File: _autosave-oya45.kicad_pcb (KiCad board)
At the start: 2 copper layers, 24 parts, among them SW1 SW_Push, U1 ATmega32U4-AU, Y1 16MHz

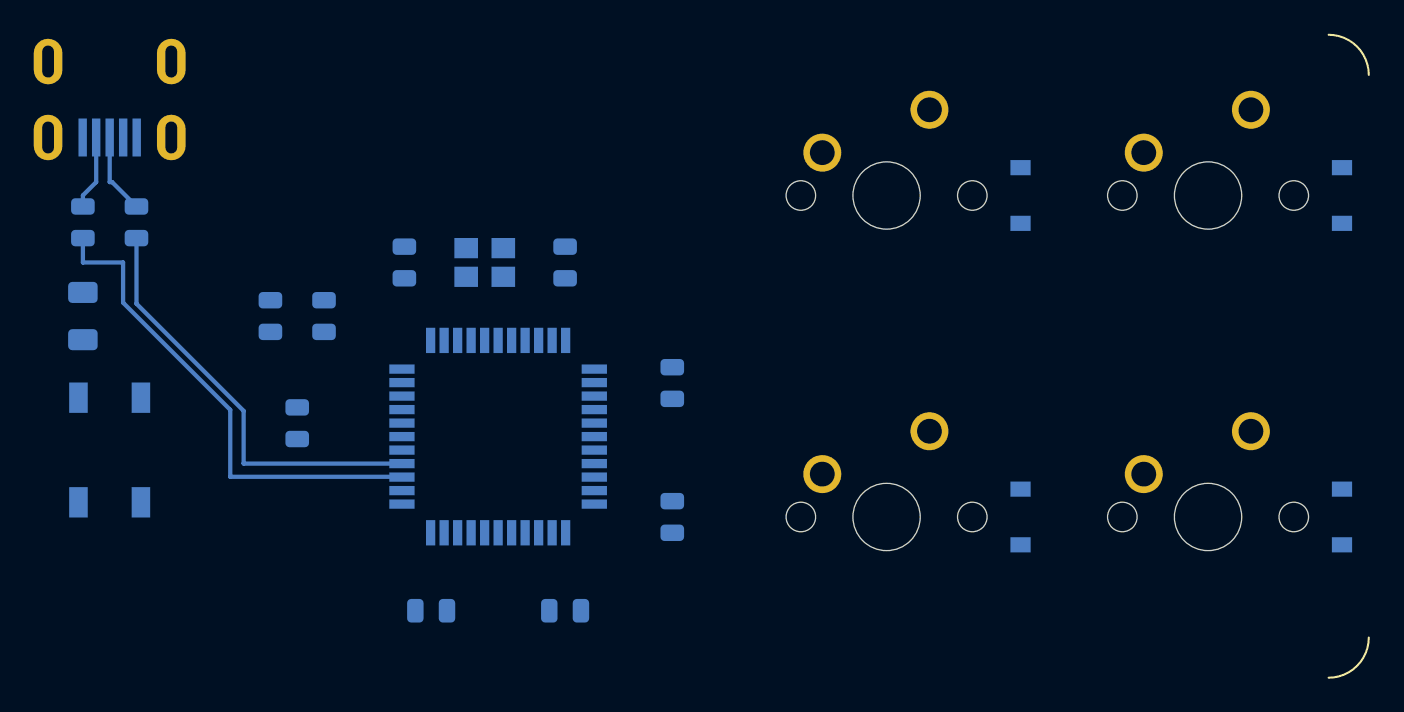
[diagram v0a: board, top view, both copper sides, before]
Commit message: test finish
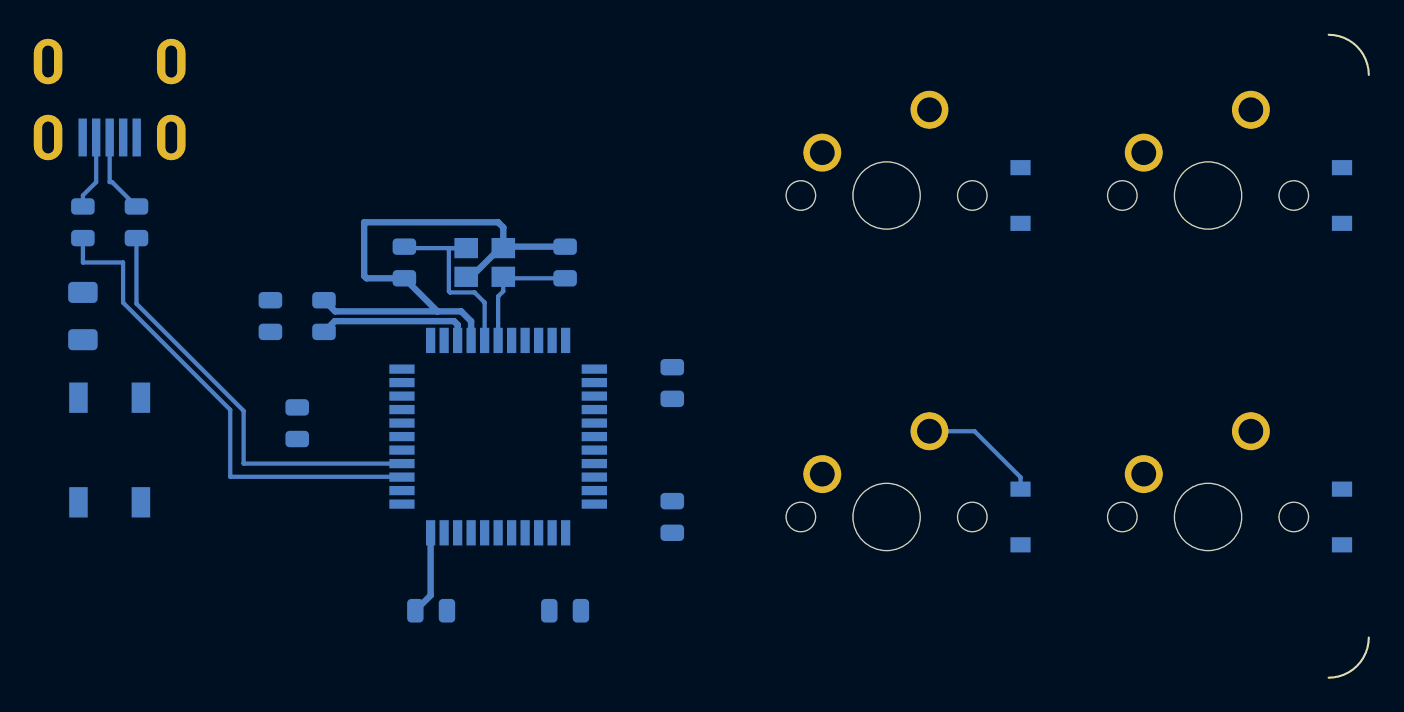
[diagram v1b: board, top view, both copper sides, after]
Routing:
- net GND: track 0.00 -> 35.0 mm
- net +5V: track 0.00 -> 14.2 mm
- net Net-(C3-Pad1): track 0.00 -> 11.9 mm
- net Net-(C2-Pad1): track 0.00 -> 7.59 mm
- net Net-(D3-Pad2): track 0.00 -> 7.23 mm
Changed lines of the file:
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@@
     (thickness 1.6)
     (drawings 2)
-    (tracks 17)
+    (tracks 58)
     (zones 0)
     (modules 24)
@@
   (gr_arc (start 194.46875 115.09375) (end 194.46875 117.475) (angle -90) (layer F.SilkS) (width 0.12))
   (gr_arc (start 194.46875 81.75625) (end 196.85 81.75625) (angle -90) (layer F.SilkS) (width 0.12))
+  (segment (start 145.5625 90.79375) (end 145.5625 92.01875) (width 0.381) (layer B.Cu) (net 1))
+  (segment (start 145.25625 90.4875) (end 145.5625 90.79375) (width 0.381) (layer B.Cu) (net 1))
+  (segment (start 137.31875 90.4875) (end 145.25625 90.4875) (width 0.381) (layer B.Cu) (net 1))
+  (segment (start 137.31875 93.6625) (end 137.31875 90.4875) (width 0.381) (layer B.Cu) (net 1))
+  (segment (start 139.7 93.80625) (end 137.4625 93.80625) (width 0.381) (layer B.Cu) (net 1))
+  (segment (start 137.4625 93.80625) (end 137.31875 93.6625) (width 0.381) (layer B.Cu) (net 1))
+  (segment (start 143.65625 96.3565) (end 143.65625 97.4875) (width 0.381) (layer B.Cu) (net 1))
+  (segment (start 145.65 91.93125) (end 145.5625 92.01875) (width 0.381) (layer B.Cu) (net 1))
+  (segment (start 149.225 91.93125) (end 145.65 91.93125) (width 0.381) (layer B.Cu) (net 1))
+  (segment (start 143.665402 93.71875) (end 143.3625 93.71875) (width 0.381) (layer B.Cu) (net 1))
+  (segment (start 145.365402 92.01875) (end 143.665402 93.71875) (width 0.381) (layer B.Cu) (net 1))
+  (segment (start 145.5625 92.01875) (end 145.365402 92.01875) (width 0.381) (layer B.Cu) (net 1))
+  (segment (start 143.065739 95.765989) (end 143.65625 96.3565) (width 0.381) (layer B.Cu) (net 1))
+  (segment (start 141.659739 95.765989) (end 143.065739 95.765989) (width 0.381) (layer B.Cu) (net 1))
+  (segment (start 139.7 93.80625) (end 141.659739 95.765989) (width 0.381) (layer B.Cu) (net 1))
+  (segment (start 135.597239 95.765989) (end 141.659739 95.765989) (width 0.381) (layer B.Cu) (net 1))
+  (segment (start 134.9375 95.10625) (end 135.597239 95.765989) (width 0.381) (layer B.Cu) (net 1))
+  (segment (start 142.85625 96.559598) (end 142.85625 97.4875) (width 0.381) (layer B.Cu) (net 2))
+  (segment (start 142.643651 96.346999) (end 142.85625 96.559598) (width 0.381) (layer B.Cu) (net 2))
+  (segment (start 135.571751 96.346999) (end 142.643651 96.346999) (width 0.381) (layer B.Cu) (net 2))
+  (segment (start 134.9375 96.98125) (end 135.571751 96.346999) (width 0.381) (layer B.Cu) (net 2))
+  (segment (start 141.25625 112.6) (end 140.35 113.50625) (width 0.381) (layer B.Cu) (net 2))
+  (segment (start 141.25625 108.8875) (end 141.25625 112.6) (width 0.381) (layer B.Cu) (net 2))
+  (segment (start 145.25625 96.4835) (end 145.25625 97.4875) (width 0.254) (layer B.Cu) (net 3))
+  (segment (start 145.25625 94.879) (end 145.25625 96.4835) (width 0.254) (layer B.Cu) (net 3))
+  (segment (start 145.5625 94.57275) (end 145.25625 94.879) (width 0.254) (layer B.Cu) (net 3))
+  (segment (start 145.5625 93.71875) (end 145.5625 94.57275) (width 0.254) (layer B.Cu) (net 3))
+  (segment (start 145.65 93.80625) (end 145.5625 93.71875) (width 0.254) (layer B.Cu) (net 3))
+  (segment (start 149.225 93.80625) (end 145.65 93.80625) (width 0.254) (layer B.Cu) (net 3))
+  (segment (start 139.7875 92.01875) (end 139.7 91.93125) (width 0.254) (layer B.Cu) (net 4))
+  (segment (start 143.3625 92.01875) (end 139.7875 92.01875) (width 0.254) (layer B.Cu) (net 4))
+  (segment (start 142.335499 94.580351) (end 142.400899 94.645751) (width 0.254) (layer B.Cu) (net 4))
+  (segment (start 142.335499 92.091751) (end 142.335499 94.580351) (width 0.254) (layer B.Cu) (net 4))
+  (segment (start 143.3625 92.01875) (end 142.4085 92.01875) (width 0.254) (layer B.Cu) (net 4))
+  (segment (start 142.4085 92.01875) (end 142.335499 92.091751) (width 0.254) (layer B.Cu) (net 4))
+  (segment (start 142.400899 94.645751) (end 143.858251 94.645751) (width 0.254) (layer B.Cu) (net 4))
+  (segment (start 144.45625 95.24375) (end 144.45625 97.4875) (width 0.254) (layer B.Cu) (net 4))
+  (segment (start 143.858251 94.645751) (end 144.45625 95.24375) (width 0.254) (layer B.Cu) (net 4))
+  (segment (start 176.2125 105.596) (end 176.2125 106.3) (width 0.254) (layer B.Cu) (net 10))
+  (segment (start 173.4865 102.87) (end 176.2125 105.596) (width 0.254) (layer B.Cu) (net 10))
+  (segment (start 170.815 102.87) (end 173.4865 102.87) (width 0.254) (layer B.Cu) (net 10))
   (segment (start 121.4375 88.10625) (end 120.65 88.89375) (width 0.254) (layer B.Cu) (net 15))
   (segment (start 121.4375 84.80625) (end 121.4375 88.10625) (width 0.254) (layer B.Cu) (net 15))
